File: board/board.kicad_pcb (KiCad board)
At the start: 2 copper layers, 21 x 13 mm, 1 part

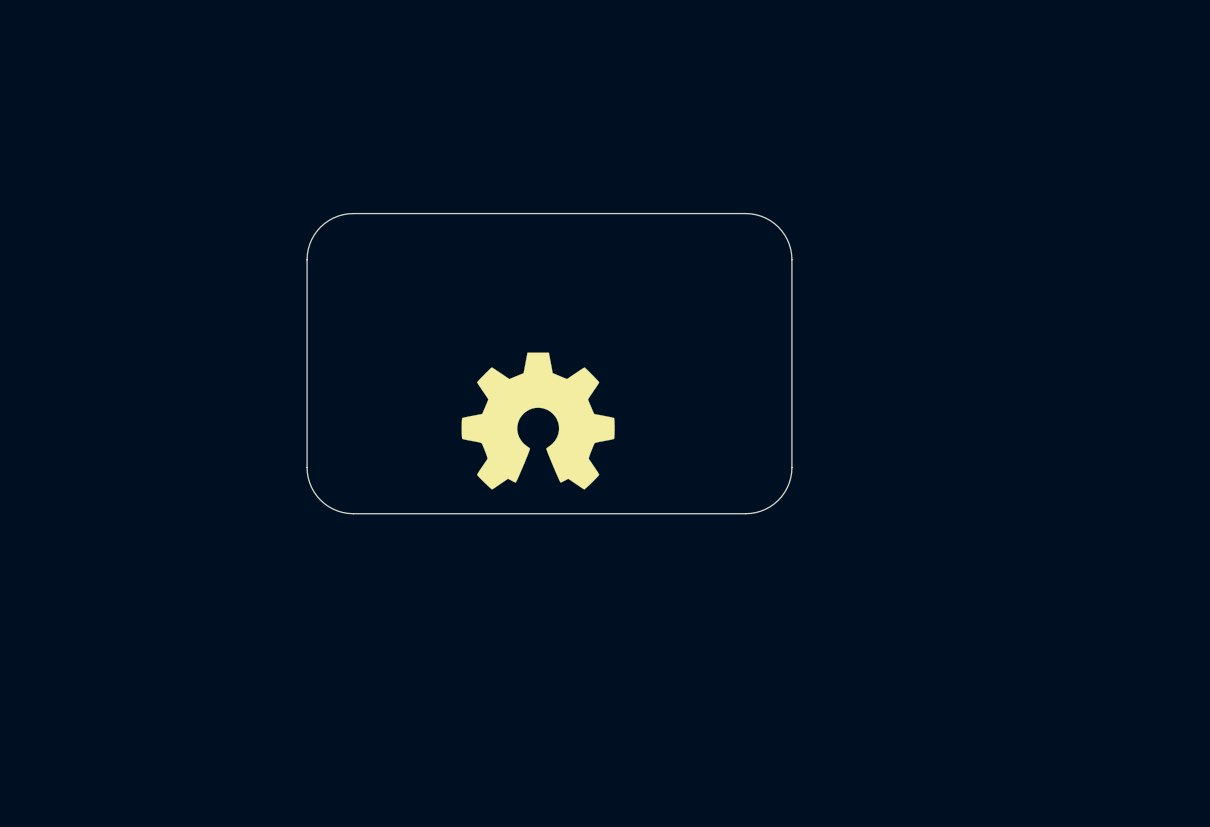
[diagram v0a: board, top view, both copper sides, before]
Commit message: initial
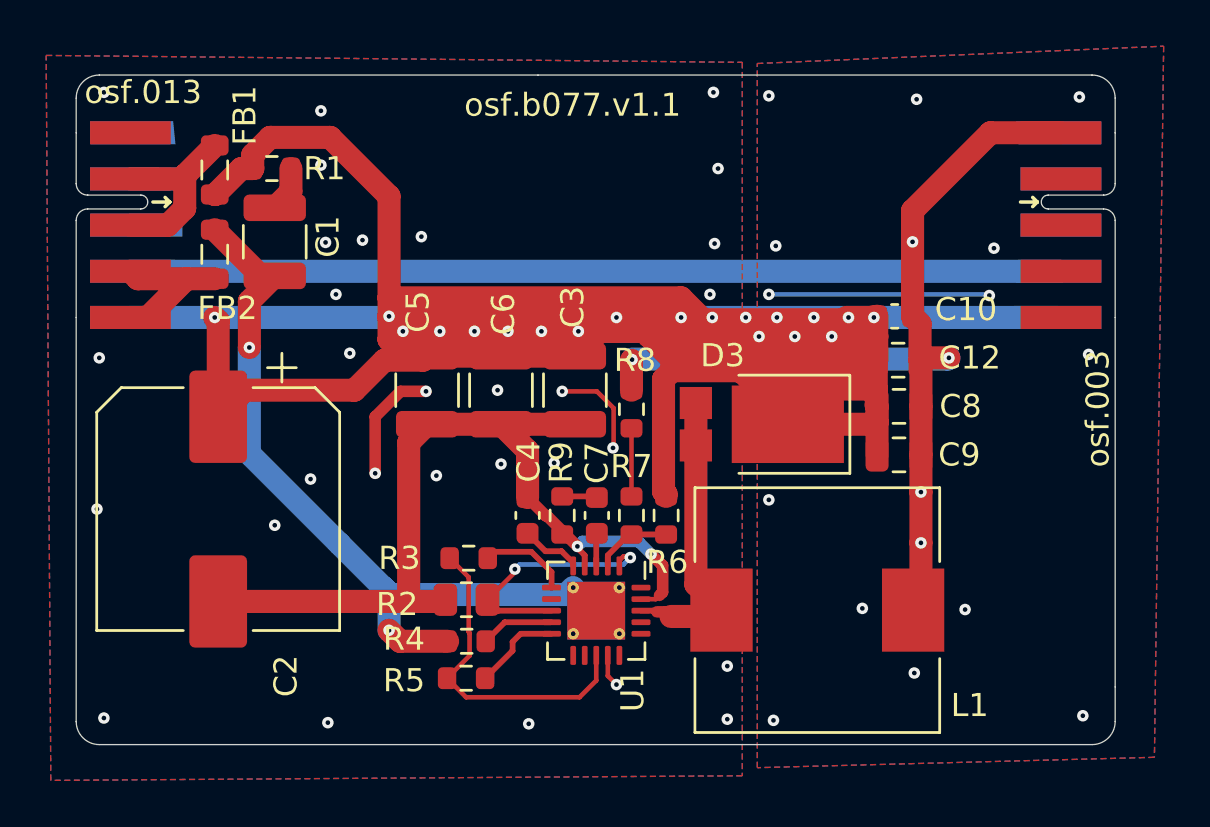
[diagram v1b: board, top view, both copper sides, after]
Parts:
- removed LOGO1: Logo_Open_Hardware_Small, Symbol:OSHW-Symbol_6.7x6mm_SilkScreen
- added C1: 100nF, Capacitor_SMD:C_1210_3225Metric, F.Cu at (138.6, 91.2)
- added C10: 1uF, Capacitor_SMD:C_0603_1608Metric, F.Cu at (165.4, 94.5)
- added C12: 100uF, Capacitor_SMD:C_0805_2012Metric, F.Cu at (165.6, 96.3)
- added C2: 10uF, Capacitor_SMD:CP_Elec_10x10, F.Cu at (136.2, 102.8)
- added C3: 1uF, Capacitor_SMD:C_1210_3225Metric, F.Cu at (151.6, 97.7)
- added C4: 100nF, Capacitor_SMD:C_0603_1608Metric, F.Cu at (149.6, 103.1)
- added C5: 100nF, Capacitor_SMD:C_1210_3225Metric, F.Cu at (145.2, 97.7)
- added C6: 10nF, Capacitor_SMD:C_1210_3225Metric, F.Cu at (148.4, 97.7)
- added C7: 330pF, Capacitor_SMD:C_0603_1608Metric, F.Cu at (152.6, 103.1)
- added C8: 100uF, Capacitor_SMD:C_0805_2012Metric, F.Cu at (165.6, 98.3)
- added C9: 100uF, Capacitor_SMD:C_0805_2012Metric, F.Cu at (165.6, 100.5)
- added D3: PDS3100, Diode_SMD:D_PowerDI-5, F.Cu at (159.7, 99.1)
- added FB1: 700R, Inductor_SMD:L_0805_2012Metric, F.Cu at (136.0, 88.1)
- added FB2: 700R, Inductor_SMD:L_0805_2012Metric, F.Cu at (136.0, 91.8)
- added J1: 013_PoE_rectified, on_edge:on_edge_2x05_device, F.Cu at (130.0, 90.5)
- added J2: 003_power, on_edge:on_edge_2x05_host, F.Cu at (175.0, 90.5)
- added L1: 47uH, Inductor_SMD:L_10.4x10.4_H4.8, F.Cu at (162.1, 107.2)
- added R1: 3R, Resistor_SMD:R_0603_1608Metric, F.Cu at (138.5, 88.0)
- added R2: 1.2R, Resistor_SMD:R_0805_2012Metric, F.Cu at (146.9, 106.7)
- added R3: 24.3k, Resistor_SMD:R_0603_1608Metric, F.Cu at (147.0, 104.9)
- added R4: 75R, Resistor_SMD:R_0603_1608Metric, F.Cu at (146.9, 108.5)
- added R5: 88.7k, Resistor_SMD:R_0603_1608Metric, F.Cu at (146.9, 110.1)
- added R6: 3.24k, Resistor_SMD:R_0603_1608Metric, F.Cu at (155.6, 103.1)
- added R7: 9.09k, Resistor_SMD:R_0603_1608Metric, F.Cu at (154.1, 103.1)
- added R8: 10R, Resistor_SMD:R_0603_1608Metric, F.Cu at (154.1, 98.5)
- added R9: 143k, Resistor_SMD:R_0603_1608Metric, F.Cu at (151.1, 103.1)
- added U1: Si3404, Package_DFN_QFN:QFN-20-1EP_4x4mm_P0.5mm_EP2.5x2.5mm_ThermalVias, F.Cu at (152.5, 107.2)
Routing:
- net /dcdc/5V: track 0.00 -> 202.2 mm, vias 0 -> 19
- net /dcdc/GND2: track 0.00 -> 51.3 mm, vias 0 -> 19
- net /dcdc/PoE-: track 0.00 -> 43.7 mm, vias 0 -> 32
- net Net-(J1-Pad9): track 0.00 -> 40.2 mm
- net VSS: track 0.00 -> 39.3 mm, vias 0 -> 2
- net Net-(D3-Pad2): track 0.00 -> 14.2 mm
- net /dcdc/VPOS: track 0.00 -> 14.2 mm
- net Net-(R2-Pad2): track 0.00 -> 10.8 mm, vias 0 -> 2
- net /dcdc/48V: track 0.00 -> 8.33 mm
- net /dcdc/GND: track 0.00 -> 6.90 mm
- net /dcdc/RDET: track 0.00 -> 3.91 mm
- net /dcdc/RFREQ: track 0.00 -> 3.90 mm
- net /dcdc/FBH: track 0.00 -> 3.36 mm
- net Net-(R4-Pad2): track 0.00 -> 3.19 mm
- net Net-(R7-Pad2): track 0.00 -> 2.95 mm
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- added copper zone on B.Cu, net /dcdc/GND2
- added copper zone on F.Cu, net /dcdc/GND2
- added copper zone on B.Cu, net /dcdc/PoE-
- added copper zone on F.Cu, net /dcdc/PoE-
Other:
- board size 21 x 13 mm -> 45 x 29 mm
- rule pad_to_mask_clearance: 0 -> 0.051
- board text added: "osf.003"
- board text added: "osf.013"
- board text added: "osf.b077.v1.1"
